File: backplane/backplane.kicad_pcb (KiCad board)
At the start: 2 copper layers, 13 parts, among them U1 PT4115

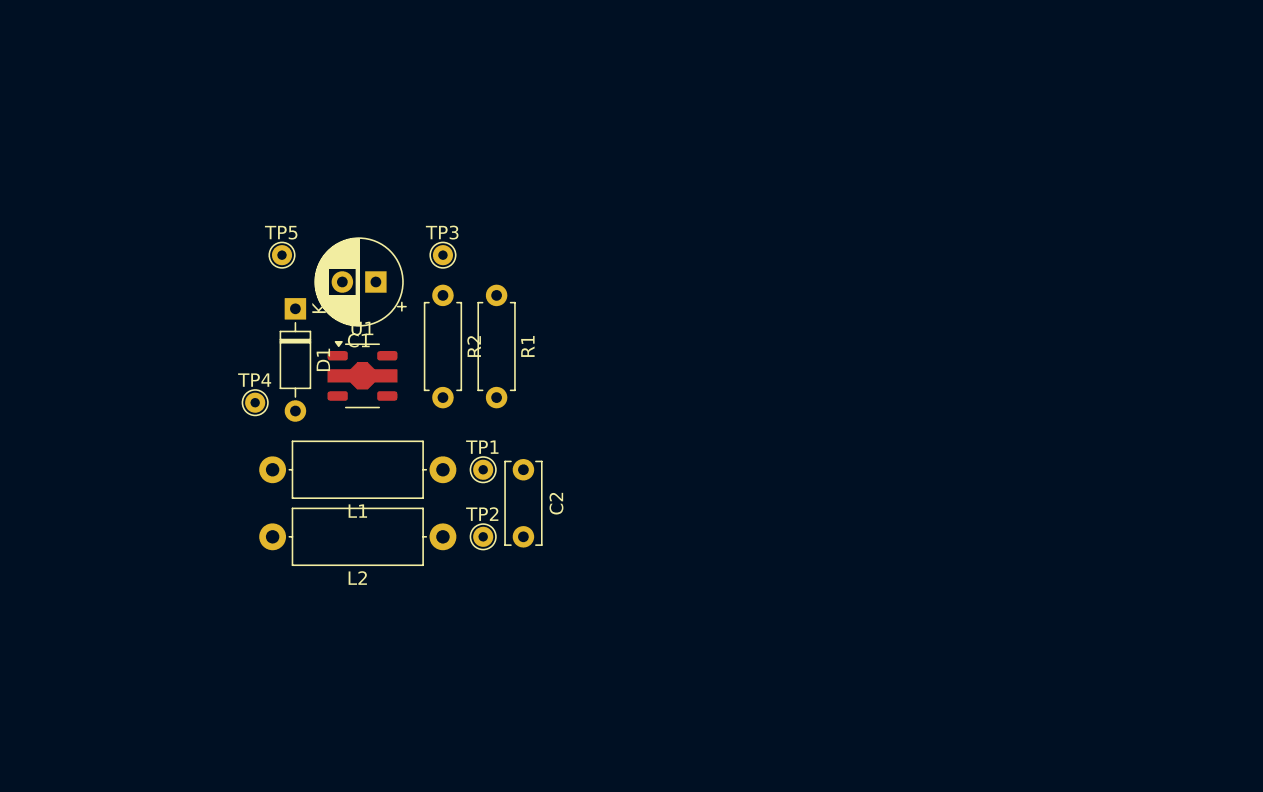
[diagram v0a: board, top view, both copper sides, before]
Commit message: Backplane work
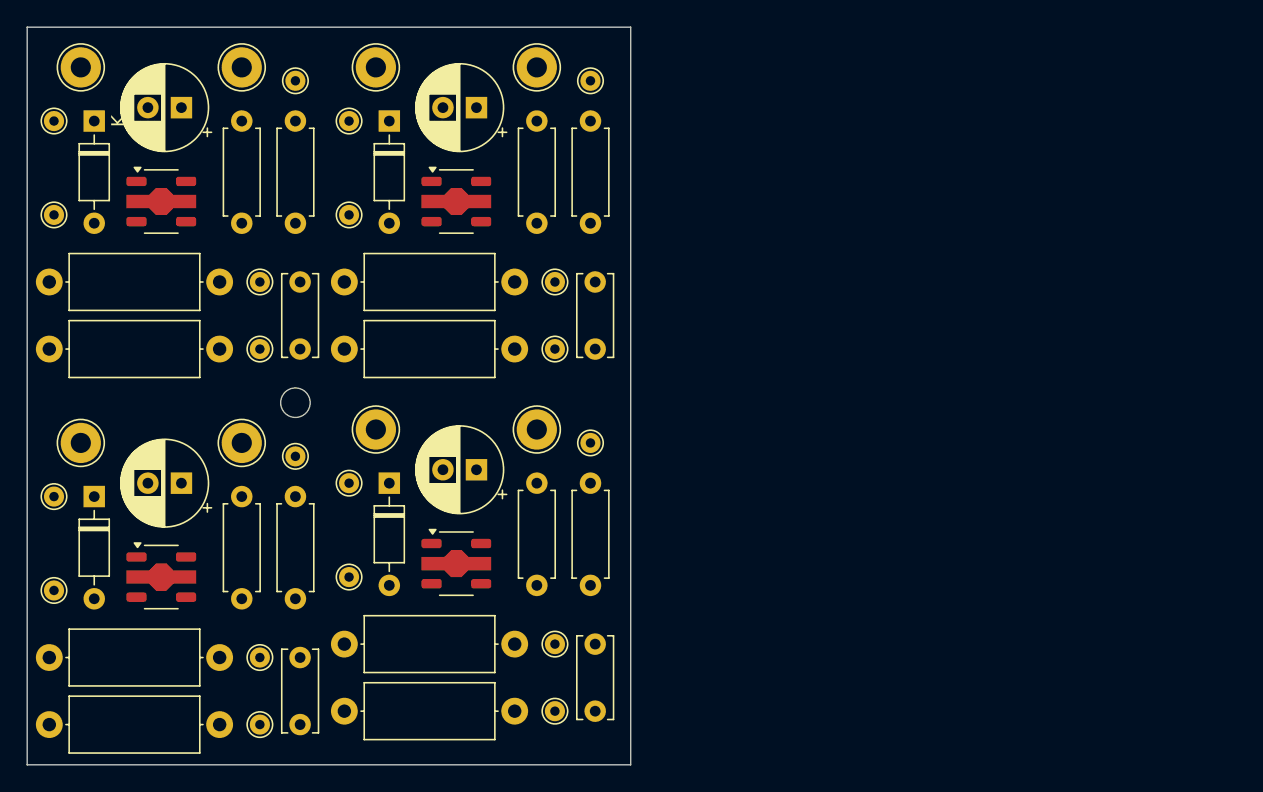
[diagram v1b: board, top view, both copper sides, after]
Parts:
- added C3: 4.7 uF - 100 uF, Capacitor_THT:CP_Radial_D6.3mm_P2.50mm, F.Cu at (33.5, 6.00)
- added C4: 0.1 uF - 1 uF, Capacitor_THT:C_Disc_D6.0mm_W2.5mm_P5.00mm, F.Cu at (42.4, 19.0)
- added C5: 4.7 uF - 100 uF, Capacitor_THT:CP_Radial_D6.3mm_P2.50mm, F.Cu at (11.5, 34.0)
- added C6: 0.1 uF - 1 uF, Capacitor_THT:C_Disc_D6.0mm_W2.5mm_P5.00mm, F.Cu at (20.4, 47.0)
- added C7: 4.7 uF - 100 uF, Capacitor_THT:CP_Radial_D6.3mm_P2.50mm, F.Cu at (33.5, 33.0)
- added C8: 0.1 uF - 1 uF, Capacitor_THT:C_Disc_D6.0mm_W2.5mm_P5.00mm, F.Cu at (42.4, 46.0)
- added D2: SR1100, Diode_THT:D_DO-35_SOD27_P7.62mm_Horizontal, F.Cu at (27.0, 7.00)
- added D3: SR1100, Diode_THT:D_DO-35_SOD27_P7.62mm_Horizontal, F.Cu at (5.00, 35.0)
- added D4: SR1100, Diode_THT:D_DO-35_SOD27_P7.62mm_Horizontal, F.Cu at (27.0, 34.0)
- added H1: MountingHole, MountingHole:MountingHole_2.2mm_M2, F.Cu at (20.0, 28.0)
- added L3: 47 uH - 100 uH, Inductor_THT:L_Axial_L9.5mm_D4.0mm_P12.70mm_Horizontal_Fastron_SMCC, F.Cu at (36.4, 19.0)
- added L4: 47 uH - 100 uH, Inductor_THT:L_Axial_L9.5mm_D4.0mm_P12.70mm_Horizontal_Fastron_SMCC, F.Cu at (36.4, 24.0)
- added L5: 47 uH - 100 uH, Inductor_THT:L_Axial_L9.5mm_D4.0mm_P12.70mm_Horizontal_Fastron_SMCC, F.Cu at (14.3, 47.0)
- added L6: 47 uH - 100 uH, Inductor_THT:L_Axial_L9.5mm_D4.0mm_P12.70mm_Horizontal_Fastron_SMCC, F.Cu at (14.3, 52.0)
- added L7: 47 uH - 100 uH, Inductor_THT:L_Axial_L9.5mm_D4.0mm_P12.70mm_Horizontal_Fastron_SMCC, F.Cu at (36.4, 46.0)
- added L8: 47 uH - 100 uH, Inductor_THT:L_Axial_L9.5mm_D4.0mm_P12.70mm_Horizontal_Fastron_SMCC, F.Cu at (36.4, 51.0)
- added R3: 3.3, Resistor_THT:R_Axial_DIN0207_L6.3mm_D2.5mm_P7.62mm_Horizontal, F.Cu at (42.0, 7.00)
- added R4: 0.15, Resistor_THT:R_Axial_DIN0207_L6.3mm_D2.5mm_P7.62mm_Horizontal, F.Cu at (38.0, 7.00)
- added R5: 3.3, Resistor_THT:R_Axial_DIN0207_L6.3mm_D2.5mm_P7.62mm_Horizontal, F.Cu at (20.0, 35.0)
- added R6: 0.15, Resistor_THT:R_Axial_DIN0207_L6.3mm_D2.5mm_P7.62mm_Horizontal, F.Cu at (16.0, 35.0)
- added R7: 3.3, Resistor_THT:R_Axial_DIN0207_L6.3mm_D2.5mm_P7.62mm_Horizontal, F.Cu at (42.0, 34.0)
- added R8: 0.15, Resistor_THT:R_Axial_DIN0207_L6.3mm_D2.5mm_P7.62mm_Horizontal, F.Cu at (38.0, 34.0)
- added TP10: TestPoint, TestPoint:TestPoint_THTPad_D1.5mm_Drill0.7mm, F.Cu at (24.0, 14.0)
- added TP11: TestPoint, TestPoint:TestPoint_THTPad_D3.0mm_Drill1.5mm, F.Cu at (26.0, 3.00)
- added TP12: TestPoint, TestPoint:TestPoint_THTPad_D1.5mm_Drill0.7mm, F.Cu at (24.0, 7.00)
- added TP13: TestPoint, TestPoint:TestPoint_THTPad_D1.5mm_Drill0.7mm, F.Cu at (39.4, 19.0)
- added TP14: TestPoint, TestPoint:TestPoint_THTPad_D1.5mm_Drill0.7mm, F.Cu at (39.4, 24.0)
- added TP15: TestPoint, TestPoint:TestPoint_THTPad_D3.0mm_Drill1.5mm, F.Cu at (16.0, 31.0)
- added TP16: TestPoint, TestPoint:TestPoint_THTPad_D1.5mm_Drill0.7mm, F.Cu at (20.0, 32.0)
- added TP17: TestPoint, TestPoint:TestPoint_THTPad_D1.5mm_Drill0.7mm, F.Cu at (2.00, 42.0)
- added TP18: TestPoint, TestPoint:TestPoint_THTPad_D3.0mm_Drill1.5mm, F.Cu at (4.00, 31.0)
- added TP19: TestPoint, TestPoint:TestPoint_THTPad_D1.5mm_Drill0.7mm, F.Cu at (2.00, 35.0)
- added TP20: TestPoint, TestPoint:TestPoint_THTPad_D1.5mm_Drill0.7mm, F.Cu at (17.4, 47.0)
- added TP21: TestPoint, TestPoint:TestPoint_THTPad_D1.5mm_Drill0.7mm, F.Cu at (17.4, 52.0)
- added TP22: TestPoint, TestPoint:TestPoint_THTPad_D3.0mm_Drill1.5mm, F.Cu at (38.0, 30.0)
- added TP23: TestPoint, TestPoint:TestPoint_THTPad_D1.5mm_Drill0.7mm, F.Cu at (42.0, 31.0)
- added TP24: TestPoint, TestPoint:TestPoint_THTPad_D1.5mm_Drill0.7mm, F.Cu at (24.0, 41.0)
- added TP25: TestPoint, TestPoint:TestPoint_THTPad_D3.0mm_Drill1.5mm, F.Cu at (26.0, 30.0)
- added TP26: TestPoint, TestPoint:TestPoint_THTPad_D1.5mm_Drill0.7mm, F.Cu at (24.0, 34.0)
- added TP27: TestPoint, TestPoint:TestPoint_THTPad_D1.5mm_Drill0.7mm, F.Cu at (39.4, 46.0)
- added TP28: TestPoint, TestPoint:TestPoint_THTPad_D1.5mm_Drill0.7mm, F.Cu at (39.4, 51.0)
- added TP6: TestPoint, TestPoint:TestPoint_THTPad_D3.0mm_Drill1.5mm, F.Cu at (16.0, 3.00)
- added TP7: TestPoint, TestPoint:TestPoint_THTPad_D3.0mm_Drill1.5mm, F.Cu at (4.00, 3.00)
- added TP8: TestPoint, TestPoint:TestPoint_THTPad_D3.0mm_Drill1.5mm, F.Cu at (38.0, 3.00)
- added TP9: TestPoint, TestPoint:TestPoint_THTPad_D1.5mm_Drill0.7mm, F.Cu at (42.0, 4.00)
- added U2: PT4115, Package_TO_SOT_SMD:SOT-89-5, F.Cu at (32.0, 13.0)
- added U3: PT4115, Package_TO_SOT_SMD:SOT-89-5, F.Cu at (10.0, 41.0)
- added U4: PT4115, Package_TO_SOT_SMD:SOT-89-5, F.Cu at (32.0, 40.0)
- R1: value 0.15 -> 3.3
- R2: value 3.3 -> 0.15
- moved TP5 40.0 mm to (2.00, 14.0)
- moved TP2 32.2 mm to (20.0, 4.00)
- moved TP3 30.7 mm to (2.00, 7.00)
- moved C2 21.8 mm to (20.4, 19.0)
- moved L1 21.8 mm to (14.3, 19.0)
- moved L2 21.8 mm to (14.3, 24.0)
- moved D1 20.5 mm to (5.00, 7.00)
- moved R1 19.8 mm to (20.0, 7.00)
- moved R2 19.8 mm to (16.0, 7.00)
- moved U1 19.8 mm to (10.0, 13.0)
- moved C1 19.5 mm to (11.5, 6.00)
- moved TP1 9.01 mm to (17.4, 19.0)
- moved TP4 7.19 mm to (17.4, 24.0)
- renumbered TP4 to TP1, TP1 to TP2, TP5 to TP4, TP2 to TP5
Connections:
- TP1 pad 1: Net-(U1-DIM) -> Net-(U1-CSN)
- TP2 pad 1: Net-(U1-CSN) -> +12V
- TP3 pad 1: +12V -> GND
- TP4 pad 1: GND -> Net-(C2-Pad2)
- TP5 pad 1: Net-(C2-Pad2) -> Net-(U1-DIM)
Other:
- board outline added: 45 x 55 mm
- rule pad_to_mask_clearance: 0 -> 0.038

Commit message: Backplane done?
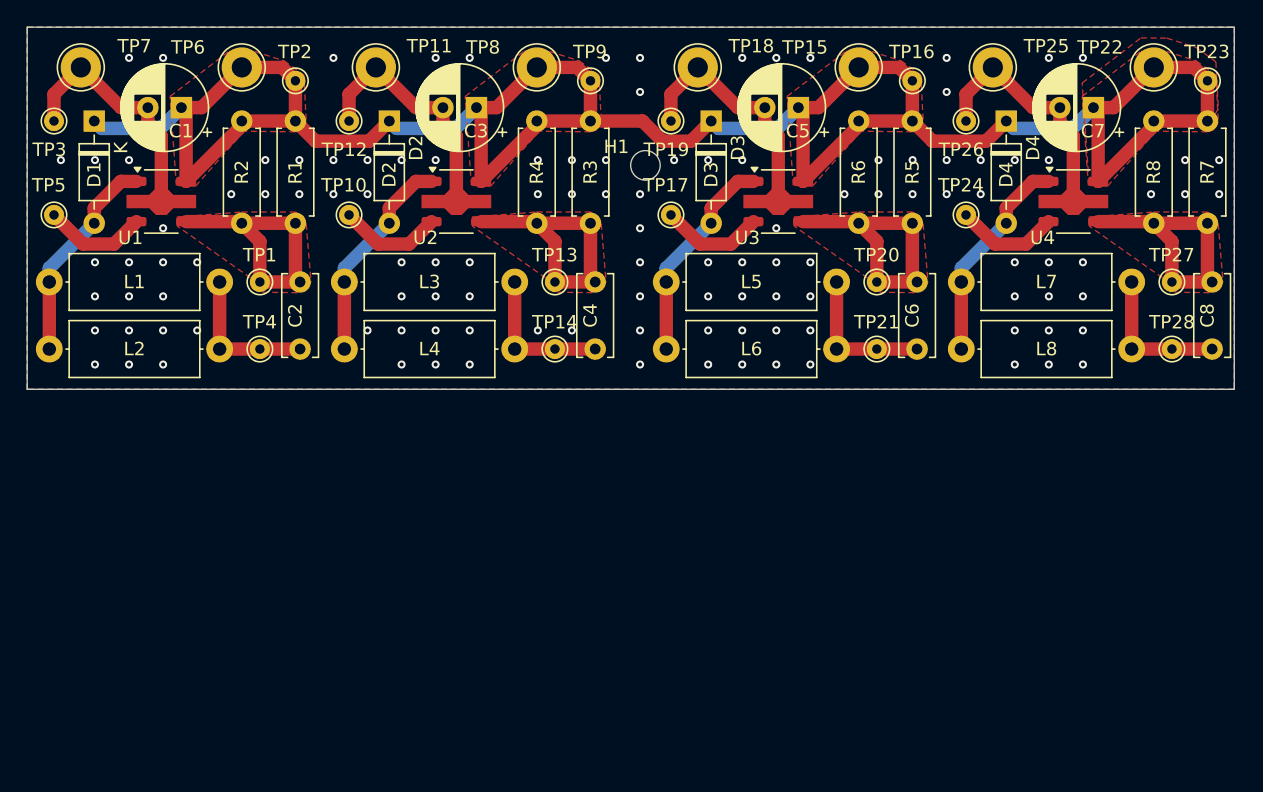
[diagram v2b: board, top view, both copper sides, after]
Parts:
- moved C5 53.9 mm to (57.5, 6.00)
- moved D3 53.9 mm to (51.0, 7.00)
- moved L5 53.9 mm to (60.4, 19.0)
- moved L6 53.9 mm to (60.4, 24.0)
- moved R5 53.9 mm to (66.0, 7.00)
- moved R6 53.9 mm to (62.0, 7.00)
- moved TP15 53.9 mm to (62.0, 3.00)
- moved TP16 53.9 mm to (66.0, 4.00)
- moved TP17 53.9 mm to (48.0, 14.0)
- moved TP18 53.9 mm to (50.0, 3.00)
- moved TP19 53.9 mm to (48.0, 7.00)
- moved TP20 53.9 mm to (63.4, 19.0)
- moved TP21 53.9 mm to (63.4, 24.0)
- moved U3 53.9 mm to (56.0, 13.0)
- moved C6 53.9 mm to (66.3, 19.0)
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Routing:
- net +12V: track 0.00 -> 172.3 mm
- net GND: track 0.00 -> 73.9 mm, vias 0 -> 119
- net Net-(U2-CSN): track 0.00 -> 20.7 mm
- net Net-(U1-CSN): track 0.00 -> 20.7 mm
- net Net-(U4-CSN): track 0.00 -> 20.7 mm
- net Net-(U3-CSN): track 0.00 -> 20.7 mm
- net Net-(D4-A): track 0.00 -> 15.9 mm
- net Net-(D3-A): track 0.00 -> 15.9 mm
- net Net-(D2-A): track 0.00 -> 15.9 mm
- net Net-(D1-A): track 0.00 -> 15.9 mm
- net Net-(C2-Pad2): track 0.00 -> 11.0 mm
- net Net-(C8-Pad2): track 0.00 -> 11.0 mm
- net Net-(C4-Pad2): track 0.00 -> 11.0 mm
- net Net-(C6-Pad2): track 0.00 -> 11.0 mm
- net Net-(U4-DIM): track 0.00 -> 7.74 mm
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- added copper zone on F.Cu, net +12V
- added copper zone on B.Cu, net GND
- added copper zone on F.Cu, net GND
- added copper zone on F.Cu, net Net-(U1-CSN)
- added copper zone on F.Cu, net Net-(U2-CSN)
- added copper zone on F.Cu, net Net-(U3-CSN)
- added copper zone on F.Cu, net Net-(U4-CSN)
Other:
- board size 45 x 55 mm -> 90 x 27 mm
